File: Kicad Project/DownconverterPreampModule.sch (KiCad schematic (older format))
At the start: 13 parts, among them U1 GALI-1+, U2 MCA1-85L+, U4 LMV751, U5 LMV751

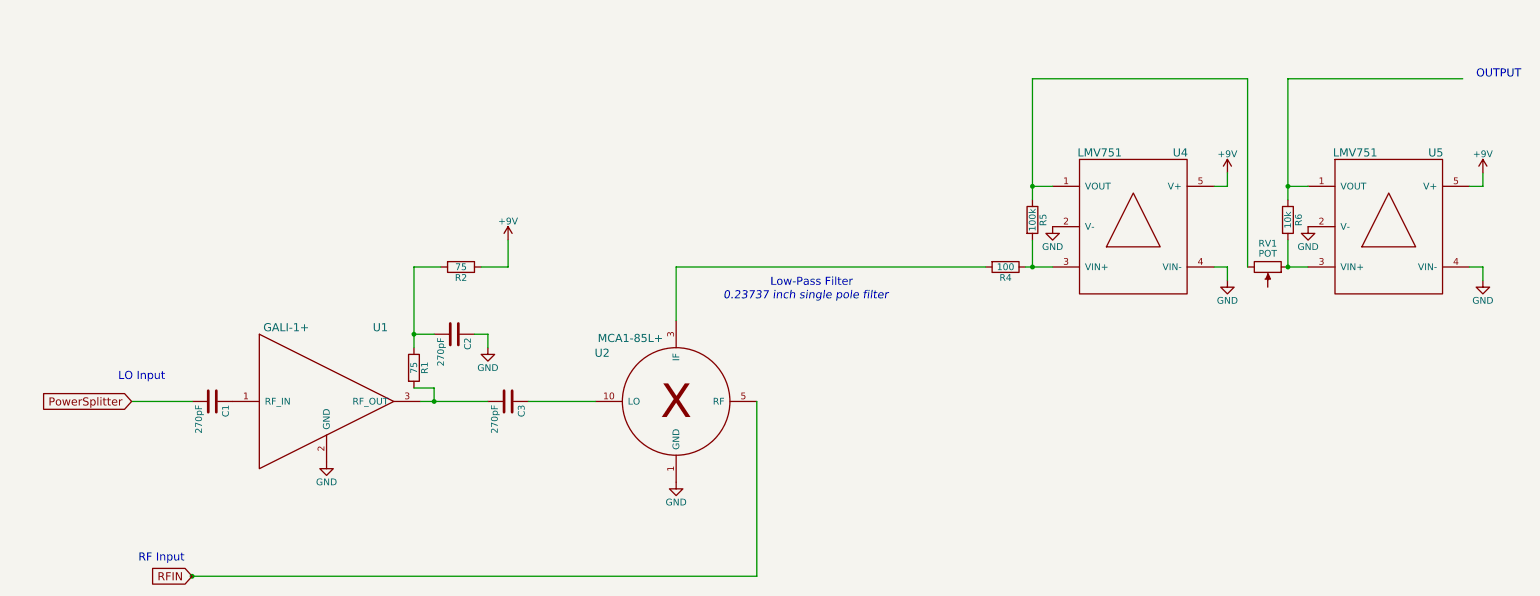
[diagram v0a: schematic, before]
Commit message: PCB
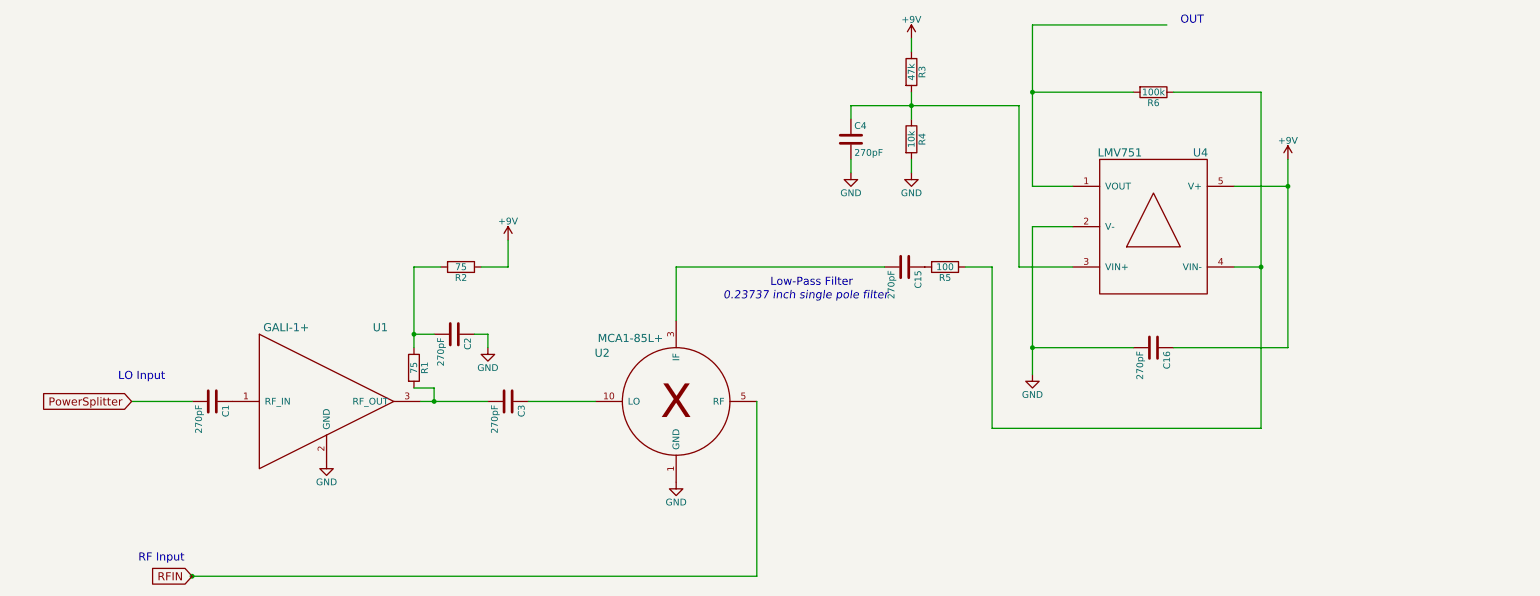
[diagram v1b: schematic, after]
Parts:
- removed RV1: POT, symbol POT
- removed U5: LMV751, RadarComponents:SOT23-5, symbol LMV751
- added C15, C16, C4: 270pF, Capacitors_SMD:C_0603, symbol C
- added R3: 47k, Resistors_SMD:R_0603, symbol R
- R4: value 100 -> 10k
- R5: value 100k -> 100
- R6: value 10k -> 100k
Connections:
- net +9V: now also C16.1, R3.1
- net GND: now also R4.2, C16.2, C4.2; no longer U4.4 (VIN-)
- net at U2.3 (IF): now also C15.2; no longer R4.2
- net at U4.1 (VOUT): now also R6.2; no longer R5.1
- net at R4.1, U4.3 (VIN+): now also C4.1, R3.2; no longer R5.2
- net at R6.1: now also R5.1, U4.4 (VIN-)
- new net: C15.1, R5.2
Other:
- note added: "OUT"
- note removed: "OUTPUT"
- moved on the sheet: U4
